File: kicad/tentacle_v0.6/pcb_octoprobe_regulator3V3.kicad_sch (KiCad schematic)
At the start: 19 parts, among them U202 AMS1117-3.3, U204 TPS2595xx, U205 TPS2595xx, U207 TPS2595xx

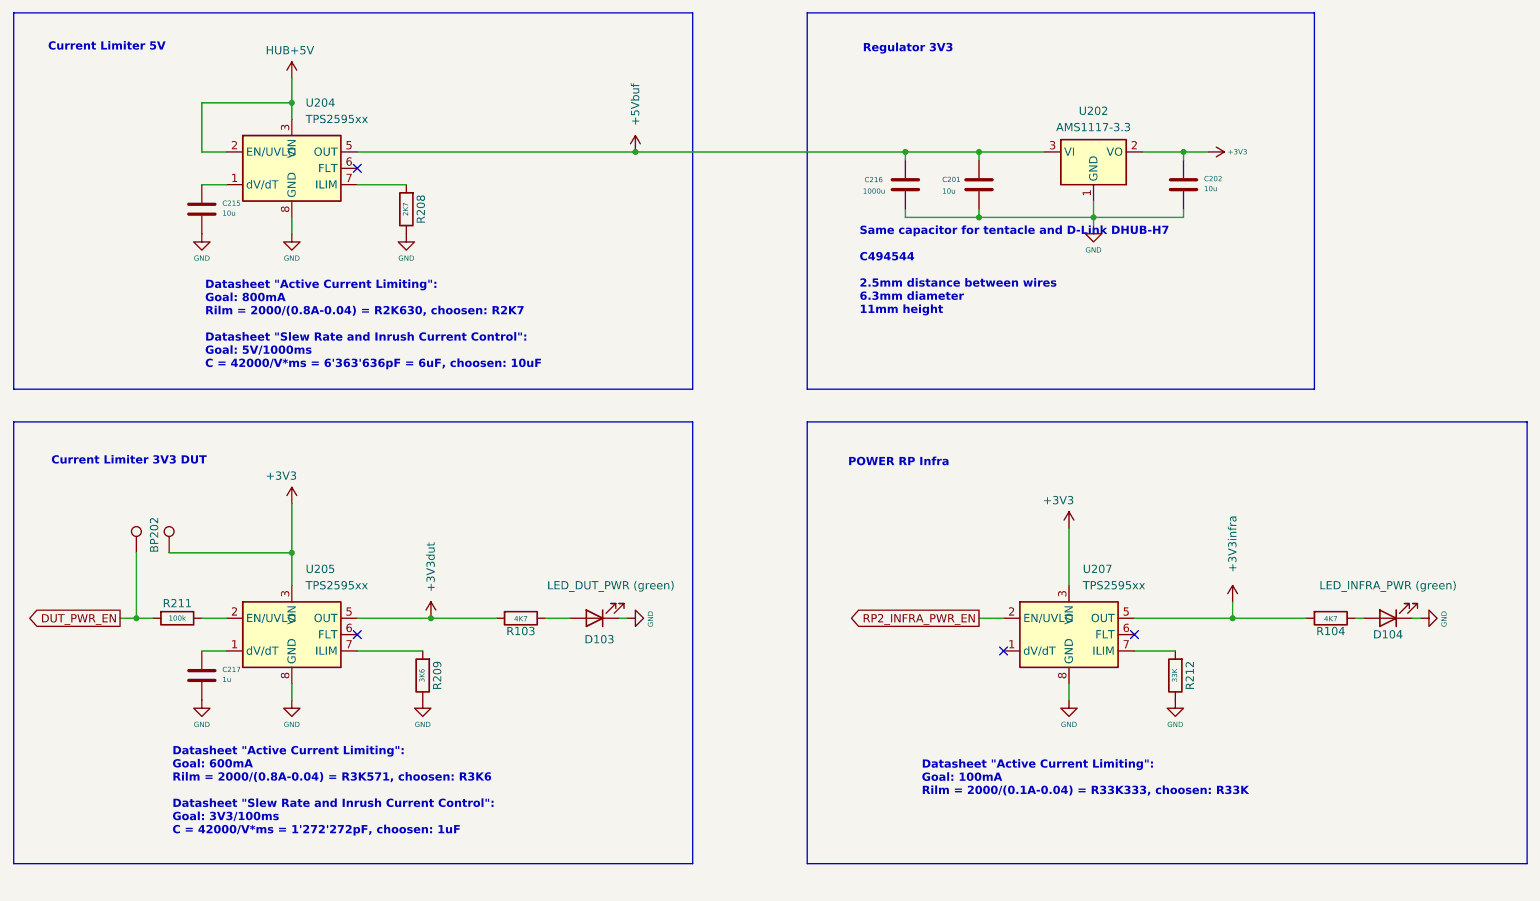
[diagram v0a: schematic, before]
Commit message: Tentacle v0.6
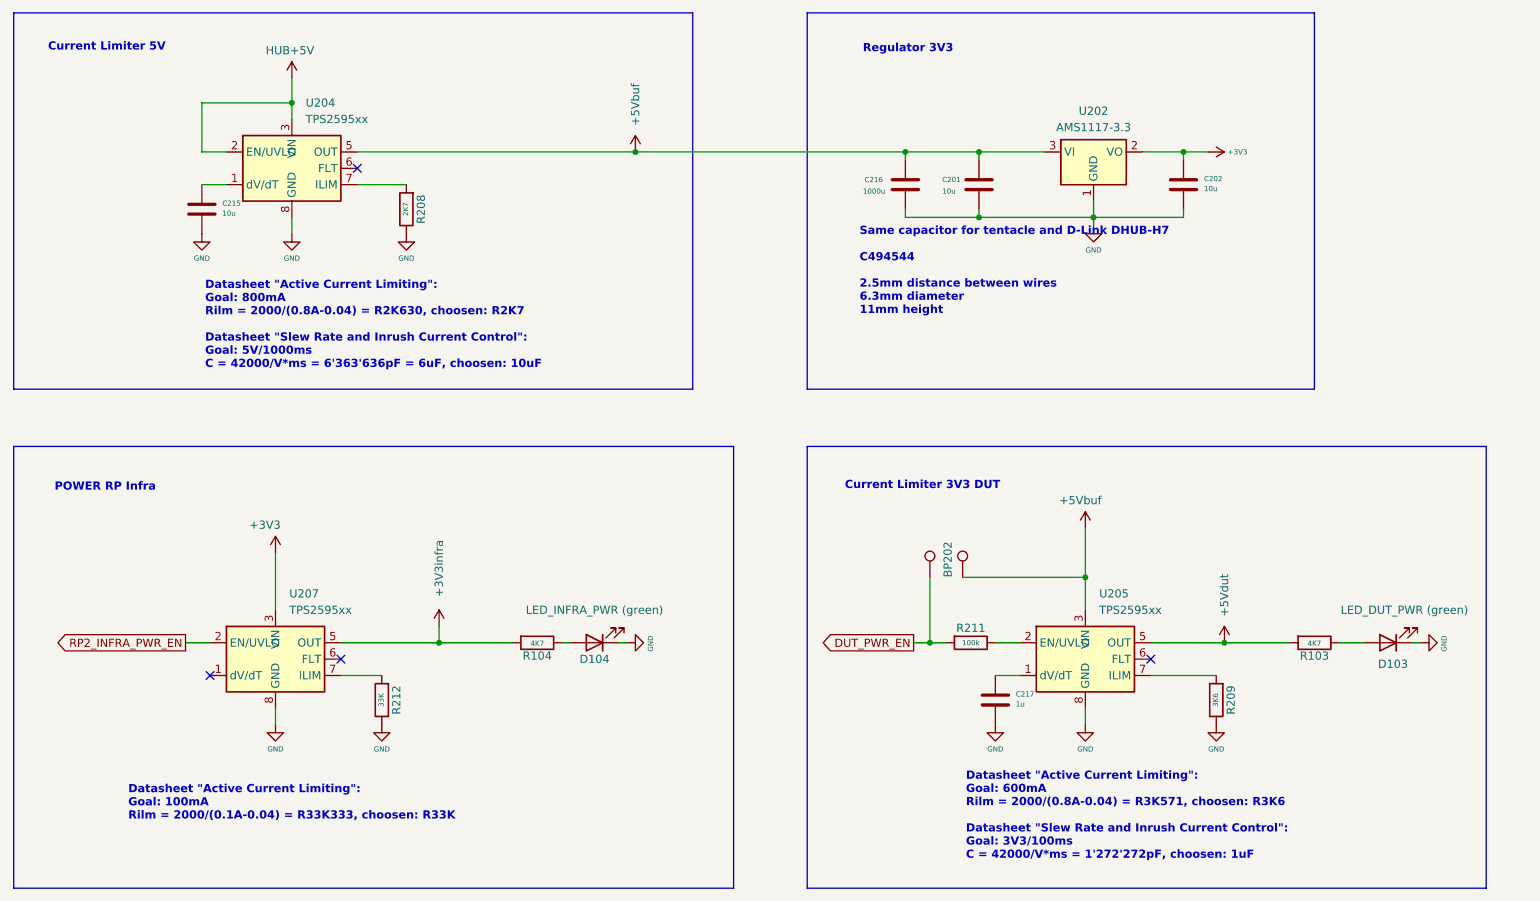
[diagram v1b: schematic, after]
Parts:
- R208, R209: footprint Resistor_SMD:R_0402_1005Metric -> Resistor_SMD:R_0603_1608Metric
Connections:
- net +3V3: no longer BP202.1, U205.3 (VIN), U205.4 (VIN)
- net +5Vbuf: now also BP202.1, U205.3 (VIN), U205.4 (VIN)
- net +3V3dut renamed +5Vdut
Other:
- moved on the sheet: BP202, C217, D103, D104, R103, R104, R209, R211, R212, U205, U207
